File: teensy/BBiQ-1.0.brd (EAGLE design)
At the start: 61.5 x 58.1 mm, 29 parts, among them IC1 ESP-WROOM-02, J1 MJ-2506N, J2 MJ-2506N, J3 MJ-2506N, J4 MJ-2506N, T1 2N3904

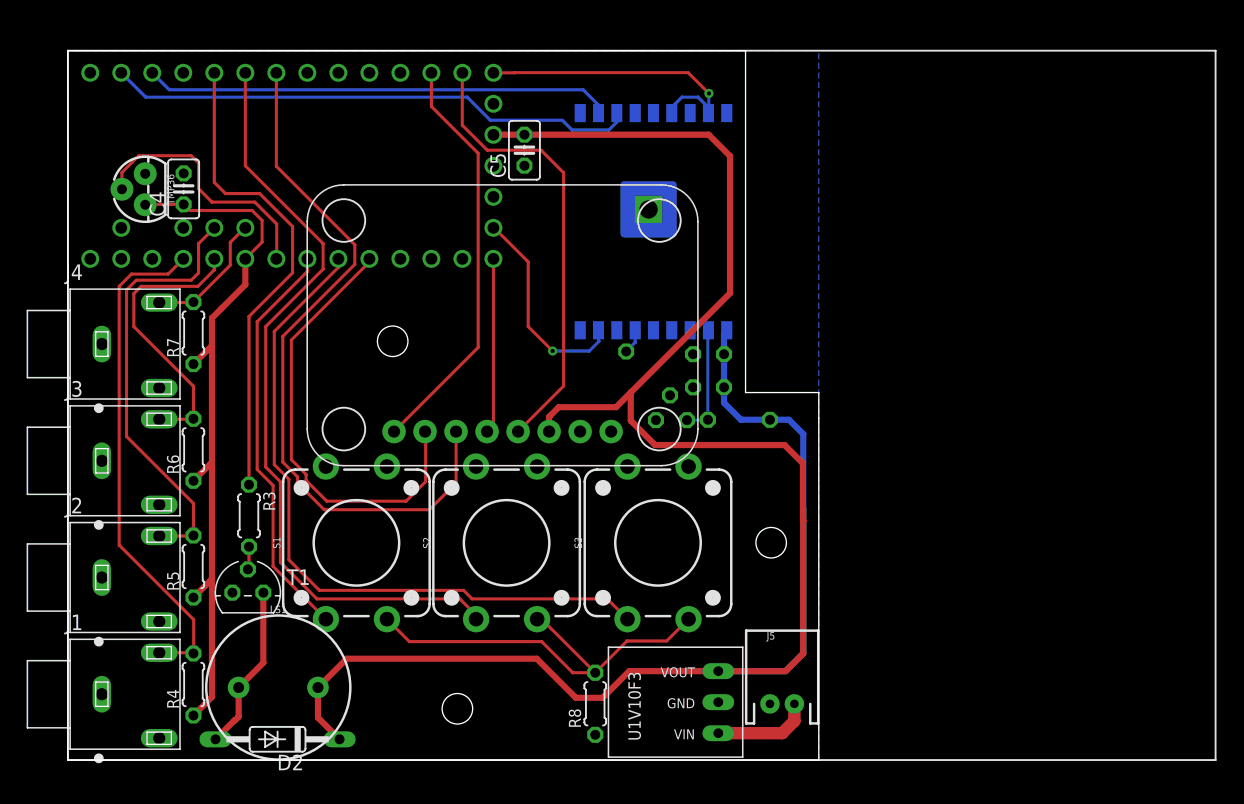
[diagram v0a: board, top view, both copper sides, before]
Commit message: New projects for final TeensyLC/ESP-WROOM-02 code
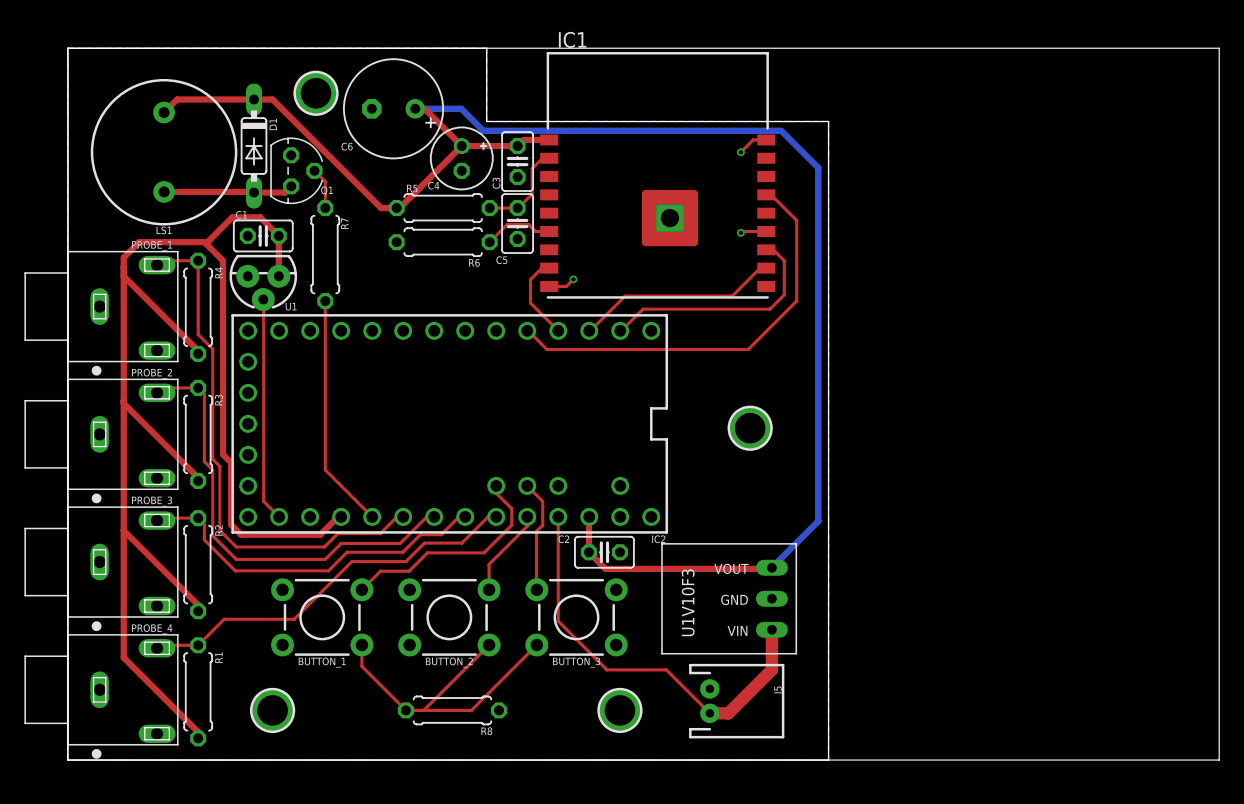
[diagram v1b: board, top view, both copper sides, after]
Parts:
- removed D2: 1N4148DO35-10, diode:DO35-10
- removed J1, J2, J3, J4: MJ-2506N, MJ-2506N:CUI_MJ-2506N
- removed OLED1: ADAFRUIT_128X32_SPI_OLED, Adafruit OLED 128x32 Mono:ADAFRUIT_128X32_SPI_OLED
- removed S1, S2, S3: MOMENTARY-SWITCH-SPST-PTH-12MM, SparkFun-Switches:TACTILE_SWITCH_PTH_12MM
- removed T1: 2N3904, transistor:TO92
- removed TMP36: (no value), SparkFun-Sensors:TO-92
- removed U$1: U1V10F3, U1V10F3:U1V10F3
- added BUTTON_1, BUTTON_2, BUTTON_3: (no value), SparkFun-Switches:TACTILE_SWITCH_PTH_6.0MM
- added C6: 1000µF, resistor:E3,5-8
- added D1: 1N4148, diode:DO35-7
- added IC2: TEENSY LC, Teensy_3_and_LC_Series_Boards_v1.4:TEENSY_3.0-3.2&LC_ALL_PINS
- added PROBE_1, PROBE_2, PROBE_3, PROBE_4: (no value), MJ-2506N:CUI_MJ-2506N
- added Q1: 2N3904, transistor:TO92
- added U$3, U$4, U$5, U$6: MOUNTINGHOLE2.5, microbuilder:MOUNTINGHOLE_2.5_PLATED
- added U1: (no value), SparkFun-Sensors:TO-92
- C1: value 10µF -> 0.1µF
- C4: value 0.1µF -> 10µF; device resistor:C025-025X050 -> resistor:E2-5
- LS1: value BUZZER-PTH -> (none)
- R1, R2, R3: value 10kΩ -> 10k 1%; device resistor:0204/5 -> resistor:0207/7
- R4: value 10kΩ 1% -> 10k 1%; device resistor:0204/5 -> resistor:0207/7
- R5, R6, R7: value 10kΩ 1% -> 10kΩ; device resistor:0204/5 -> resistor:0207/7
- R8: value 1kΩ -> 10k 1%; device resistor:0204/5 -> resistor:0207/7
- U$2: value TEENSY_LC_ALL_PINS -> U1V10F3; device Teensy_3_and_LC_Series_Boards_v1.4:TEENSY_3.0-3.2&LC_ALL_PINS -> U1V10F3:U1V10F3
- moved U$2 52.9 mm to (57.7, 13.2), flipped to the top, turned to 90 degrees
- moved R1 49.6 mm to (10.7, 5.59), flipped to the top, turned to 270 degrees
- moved LS1 44.8 mm to (7.87, 49.8), turned to 270 degrees
- moved R2 40.0 mm to (10.7, 16.0), flipped to the top, turned to 270 degrees
- moved C1 38.5 mm to (16.0, 42.9), flipped to the top, turned to 180 degrees
- moved R5 35.8 mm to (30.7, 45.2), turned to 180 degrees
- moved R4 30.9 mm to (10.7, 37.1), turned to 270 degrees
- moved R6 26.6 mm to (30.7, 42.4), turned to 180 degrees
- moved C3 24.6 mm to (36.8, 49.0), flipped to the top, turned to 270 degrees
- moved C4 22.9 mm to (32.3, 49.3), turned to 270 degrees
- moved C2 18.3 mm to (43.9, 17.0), flipped to the top
- moved R7 12.6 mm to (21.1, 41.4)
- moved R8 11.7 mm to (31.5, 4.06), turned to 180 degrees
- moved R3 7.85 mm to (10.7, 26.7)
- moved C5 6.03 mm to (36.8, 43.9), turned to 270 degrees
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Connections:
- removed net 3V3O: OLED1.7
- removed net BUTTON_0: S1.3, S1.4, U$2.19/A5
- removed net ESP_LOAD: IC1.8, U$2.RESET/DAC
- removed net N$6: D2.A, LS1.-, T1.1
- removed net N$7: R8.2, S1.1, S1.2, S2.1, S2.2, S3.1, S3.2
- removed net OLED_CK: OLED1.4, U$2.13
- removed net PROBE_0: J1.2, R4.2, U$2.23/A9
- removed net TMP36: TMP36.2, U$2.20/A6
- new net 26/A12/DAC: IC2.RESET/DAC
- new net BUTTON_3: BUTTON_3.1, IC2.A10
- new net ESP_EN: C5.1, IC1.2, R5.1
- new net ESP_PRG: IC1.8, IC2.2
- new net INT_TEMP: IC2.14/A0, U1.2
- new net N$1: IC1.6, R6.1
- new net OLED_SCLK: IC2.13
- new net PROBE_4: IC2.21/A7, PROBE_4.2, R1.1
- net +3V3: now also C3.1, C4.+, C6.+, D1.C, IC2.3.3V, IC2.3.3V1, LS1.-, R5.2, U$2.VOUT; no longer C1.1, C5.2, D2.C, LS1.+, OLED1.6, R1.2, U$1.VOUT, U$2.3.3V, U$2.3.3V1
- net AREF: now also IC2.AREF; no longer U$2.AREF
- net BUTTON_1: now also BUTTON_1.3, IC2.A11; no longer S2.3, S2.4, U$2.4
- net BUTTON_2: now also BUTTON_2.3, IC2.22/A8; no longer S3.3, S3.4, U$2.18/A4
- net BUZZER: now also IC2.17/A3, R7.1; no longer R3.1, U$2.3
- net ESP_RST: now also IC2.3; no longer IC1.17, U$2.12
- net ESP_RX: now also IC2.1; no longer U$2.1
- net ESP_TX: now also IC2.0; no longer U$2.0
- net GND: now also C3.2, C4.-, C5.2, C6.-, IC2.AGND, IC2.GND, IC2.GND1, PROBE_1.1, PROBE_1.3, PROBE_2.3, PROBE_3.1, PROBE_3.3, PROBE_4.1, PROBE_4.3, Q1.3, R6.2, U1.3; no longer C3.1, C4.2, C5.1, J1.1, J1.3, J2.1, J2.3, J3.1, J3.3, J4.1, J4.3, OLED1.8, R2.1, T1.3, TMP36.3, U$1.GND, U$2.AGND, U$2.GND1
- net N$2: now also Q1.2, R7.2; no longer C3.2, IC1.2, R1.1
- net N$3: now also D1.A, LS1.+, Q1.1; no longer IC1.6, R2.2
- net N$4: now also BUTTON_1.1, BUTTON_2.1, BUTTON_3.3, R8.2; no longer R3.2, T1.2
- net OLED_CS: now also IC2.10; no longer OLED1.1, U$2.10
- net OLED_DATA: now also IC2.11; no longer OLED1.5, U$2.11
- net OLED_DC: now also IC2.5; no longer OLED1.3, U$2.5
- net OLED_RST: now also IC2.15/A1; no longer OLED1.2, U$2.17/A3
- net PROBE_1: now also IC2.18/A4, PROBE_1.2, R4.1; no longer J2.2, R5.2, U$2.A10
- net PROBE_2: now also IC2.19/A5, PROBE_2.2, R3.1; no longer J3.2, R6.2, U$2.22/A8
- net PROBE_3: now also IC2.20/A6, PROBE_3.2, R2.1; no longer J4.2, R7.2, U$2.A11
- net PROBE_PWR: now also C1.1, IC2.16/A2, R1.2, R2.2, R3.2, R4.2, U1.1; no longer C4.1, R4.1, R5.1, R6.1, R7.1, TMP36.1, U$2.21/A7
- net VBAT: now also IC2.23/A9, U$2.VIN; no longer U$1.VIN
- net VIN: now also IC2.VIN; no longer U$2.VIN
- net VUSB: now also IC2.VUSB; no longer U$2.VUSB
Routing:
- net PROBE_PWR: track 59.7 -> 121.8 mm
- net OLED_DC: track 58.2 -> 0.00 mm
- net BUTTON_2: track 57.1 -> 7.26 mm
- net BUTTON_1: track 63.3 -> 18.2 mm
- net +3V3: track 173.8 -> 130.9 mm
- net PROBE_0: track 41.6 -> 0.00 mm
- net OLED_DATA: track 37.0 -> 0.00 mm
- net OLED_RST: track 36.6 -> 0.00 mm
- net N$7: track 34.9 -> 0.00 mm
- net OLED_CS: track 33.8 -> 0.00 mm
- net BUTTON_0: track 33.5 -> 0.00 mm
- net PROBE_4: track 0.00 -> 32.2 mm
- net N$4: track 1.89 -> 28.8 mm
- net VBAT: track 8.04 -> 33.9 mm
- net ESP_TX: track 43.5 -> 19.3 mm
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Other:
- board size 61.5 x 58.1 mm -> 62.3 x 58.3 mm
